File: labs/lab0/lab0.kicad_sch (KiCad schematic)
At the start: 6 parts, among them J1 Conn_01x02_Pin, J2 Conn_01x02_Pin

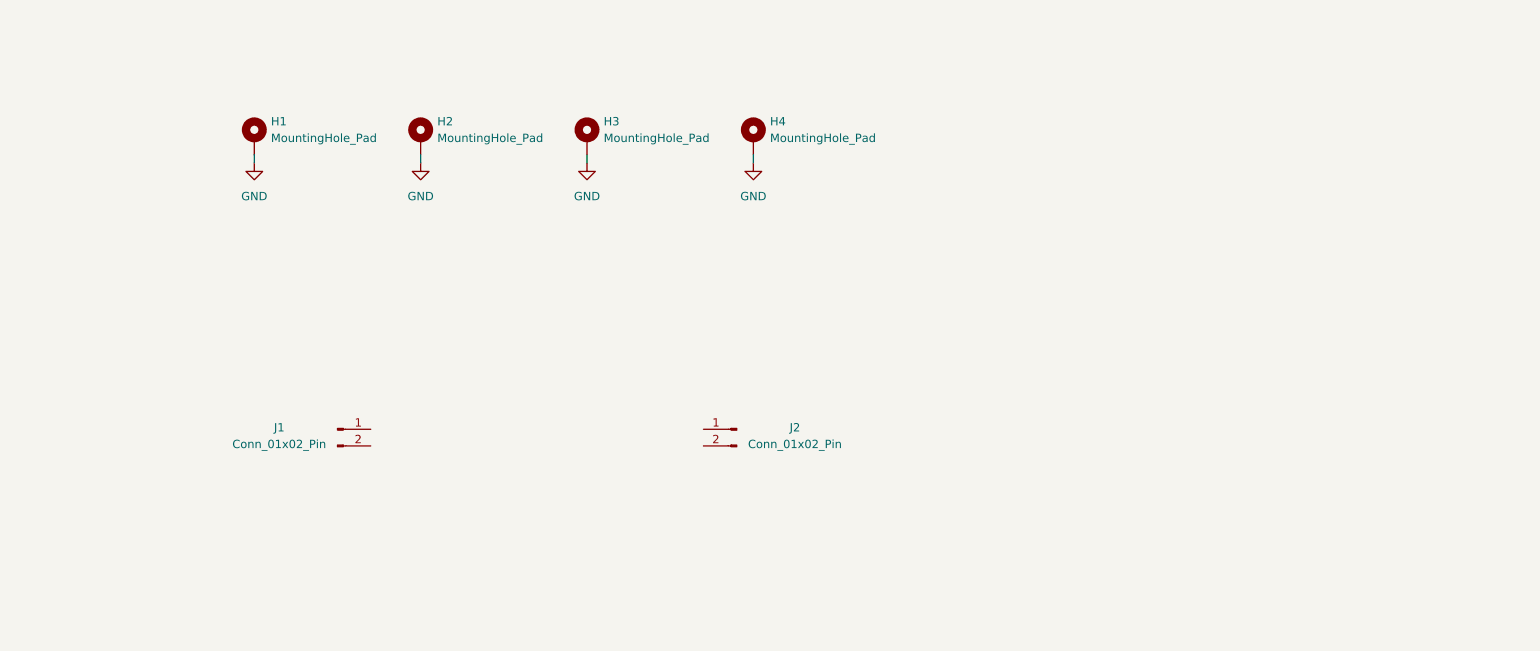
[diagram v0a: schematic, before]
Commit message: lab0 finished
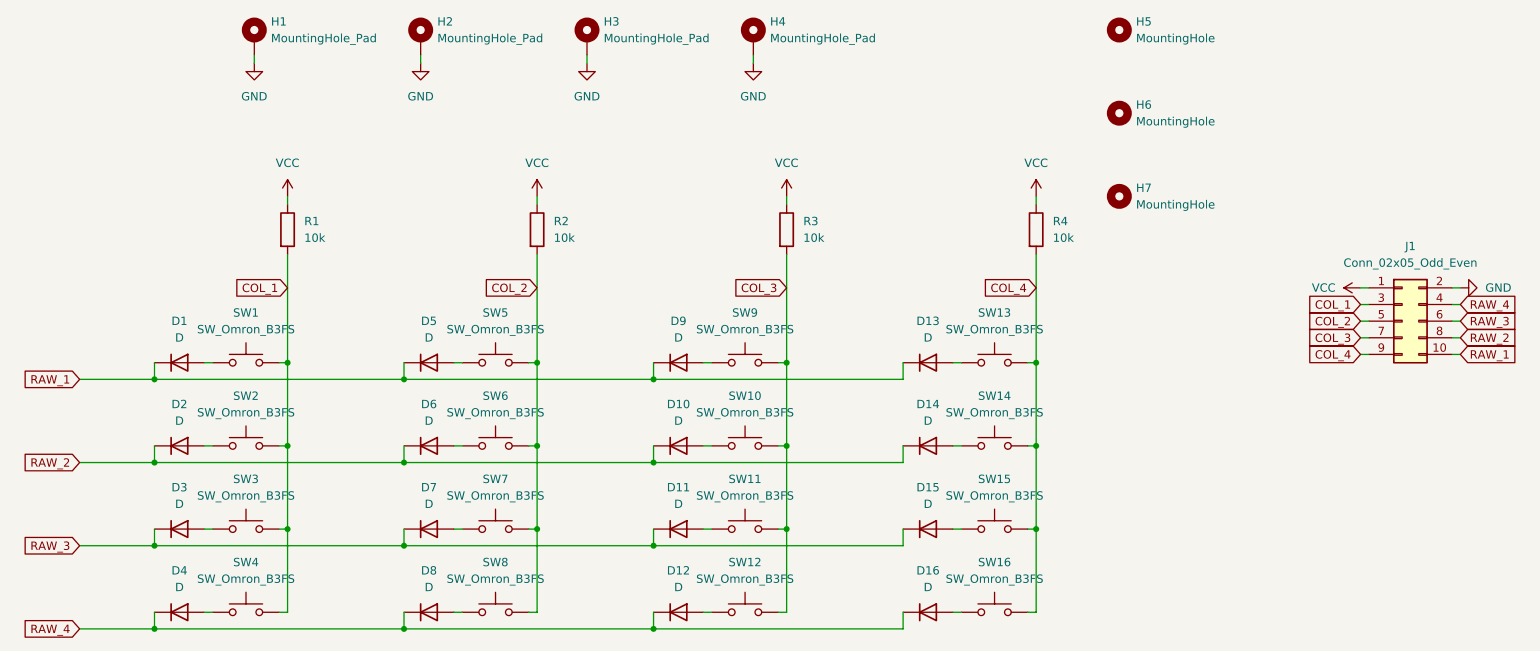
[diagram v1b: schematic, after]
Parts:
- removed J1, J2: Conn_01x02_Pin, Connector_Phoenix_GMSTB:PhoenixContact_GMSTBA_2,5_2-G-7,62_1x02_P7.62mm_Horizontal, symbol Connector:Conn_01x02_Pin
- added D1, D10, D11, D12, D13, D14, D15, D16, D2, D3, D4, D5, D6, D7, D8, D9: D, Diode_SMD:D_0603_1608Metric, symbol Device:D
- added H5, H6, H7: MountingHole, MountingHole:ToolingHole_1.152mm, symbol Mechanical:MountingHole
- added J1: Conn_02x05_Odd_Even, Connector_PinHeader_2.54mm:PinHeader_2x05_P2.54mm_Vertical, symbol Connector_Generic:Conn_02x05_Odd_Even
- added R1, R2, R3, R4: 10k, Resistor_SMD:R_0603_1608Metric, symbol Device:R
- added SW1, SW10, SW11, SW12, SW13, SW14, SW15, SW16, SW2, SW3, SW4, SW5, SW6, SW7, SW8, SW9: SW_Omron_B3FS, Button_Switch_THT:SW_PUSH_6mm, symbol Switch:SW_Omron_B3FS
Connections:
- net GND: now also J1.2 (Pin_2)
- new net: D5.2 (A), SW5.1
- new net: D7.2 (A), SW7.1
- new net: D4.2 (A), SW4.1
- new net: D15.2 (A), SW15.1
- new net: D10.2 (A), SW10.1
- new net: D9.2 (A), SW9.1
- new net: D14.2 (A), SW14.1
- new net: D3.2 (A), SW3.1
- new net: D6.2 (A), SW6.1
- new net: D13.2 (A), SW13.1
- new net: D11.2 (A), SW11.1
- new net: D16.2 (A), SW16.1
- new net: D2.2 (A), SW2.1
- new net: D8.2 (A), SW8.1
- new net: D12.2 (A), SW12.1
- new net: D1.2 (A), SW1.1
- new net COL_1: J1.3 (Pin_3), R1.2, SW1.2, SW2.2, SW3.2, SW4.2
- new net COL_2: J1.5 (Pin_5), R2.2, SW5.2, SW6.2, SW7.2, SW8.2
- new net COL_3: J1.7 (Pin_7), R3.2, SW10.2, SW11.2, SW12.2, SW9.2
- new net COL_4: J1.9 (Pin_9), R4.2, SW13.2, SW14.2, SW15.2, SW16.2
- new net RAW_1: D1.1 (K), D13.1 (K), D5.1 (K), D9.1 (K), J1.10 (Pin_10)
- new net RAW_2: D10.1 (K), D14.1 (K), D2.1 (K), D6.1 (K), J1.8 (Pin_8)
- new net RAW_3: D11.1 (K), D15.1 (K), D3.1 (K), D7.1 (K), J1.6 (Pin_6)
- new net RAW_4: D12.1 (K), D16.1 (K), D4.1 (K), D8.1 (K), J1.4 (Pin_4)
- new net VCC: J1.1 (Pin_1), R1.1, R2.1, R3.1, R4.1
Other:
- company: (none) -> TEST
- title: (none) -> Keypab_Lab0
- moved on the sheet: H1, H2, H3, H4
